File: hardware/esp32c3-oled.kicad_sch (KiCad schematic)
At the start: 2 parts, among them U1 ESP32-C3-WROOM-02

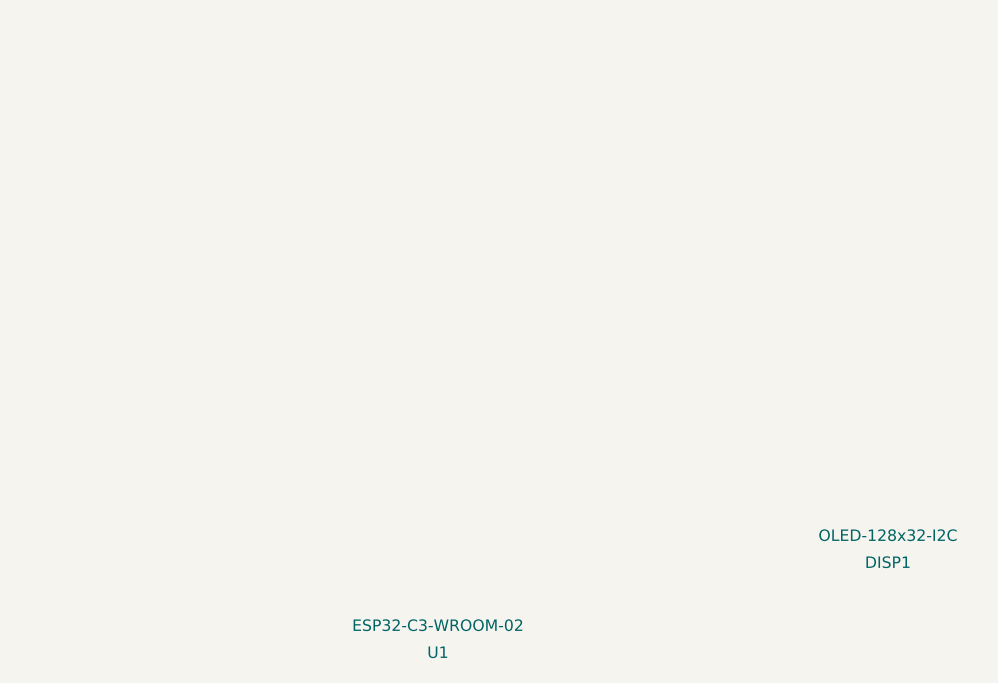
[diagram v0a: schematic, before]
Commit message: Update KiCad files
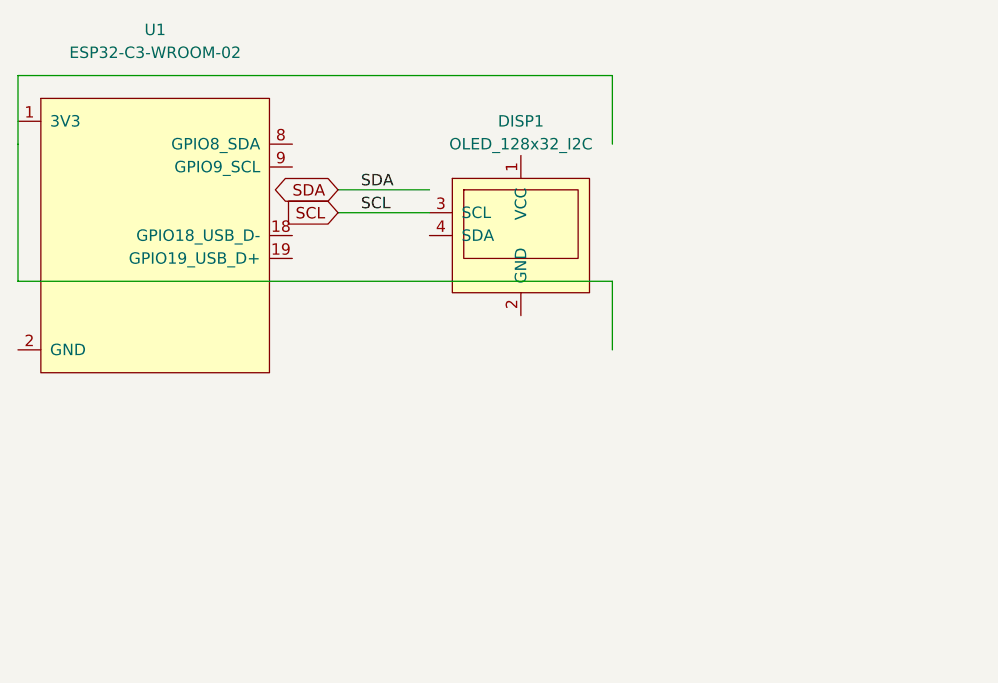
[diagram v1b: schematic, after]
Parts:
- DISP1: value OLED-128x32-I2C -> OLED_128x32_I2C; symbol Display_Character:OLED-128x32-I2C -> Display:OLED_128x32_I2C
- U1: symbol MCU_Module:ESP32-C3-WROOM-02 -> ESP32-C3:ESP32-C3-WROOM-02
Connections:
- new net SCL: DISP1.3 (SCL)
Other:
- title: (none) -> ESP32-C3 OLED Display - LCD4Linux
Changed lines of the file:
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@@
-(kicad_sch (version 20211123) (generator eeschema)
+(kicad_sch (version 20230121) (generator eeschema)
   (paper "A4")
-  (title "ESP32-C3 OLED Display - LCD4Linux")
-  (date "2026-03-09")
-  (rev "1.0")
-  (company "")
-  (comment 1 "128x32 I2C OLED with ESP32-C3")
-  (comment 2 "USB Serial communication for LCD4Linux")
-  (comment 3 "")
-  (comment 4 "")
-  (symbol (lib_id "MCU_Module:ESP32-C3-WROOM-02") (at 100 100 0) (unit 1)
-    (in_bom yes) (on_board yes)
-    (property "Reference" "U1" (id 0) (at 100 120 0))
-    (property "Value" "ESP32-C3-WROOM-02" (id 1) (at 100 117 0))
+  (title_block
+    (title "ESP32-C3 OLED Display - LCD4Linux")
+    (date "2026-03-12")
+    (rev "1.0")
+    (company "")
+    (comment 1 "128x32 I2C OLED with ESP32-C3")
+    (comment 2 "USB Serial communication for LCD4Linux")
+    (comment 3 "")
+    (comment 4 "")
   )
-  (symbol (lib_id "Display_Character:OLED-128x32-I2C") (at 150 100 0) (unit 1)
-    (in_bom yes) (on_board yes)
-    (property "Reference" "DISP1" (id 0) (at 150 110 0))
-    (property "Value" "OLED-128x32-I2C" (id 1) (at 150 107 0))
+  (wire (pts (xy 88.9 68.58) (xy 99.06 68.58))
+    (stroke (width 0) (type default))
+  )
+  (wire (pts (xy 88.9 71.12) (xy 99.06 71.12))
+    (stroke (width 0) (type default))
+  )
+  (wire (pts (xy 53.34 63.5) (xy 53.34 78.74))
+    (stroke (width 0) (type default))
+  )
+  (wire (pts (xy 119.38 78.74) (xy 119.38 86.36))
+    (stroke (width 0) (type default))
+  )
+  (wire (pts (xy 53.34 78.74) (xy 119.38 78.74))
+    (stroke (width 0) (type default))
+  )
+  (wire (pts (xy 53.34 55.88) (xy 53.34 63.5))
+    (stroke (width 0) (type default))
+  )
+  (wire (pts (xy 119.38 55.88) (xy 119.38 63.5))
+    (stroke (width 0) (type default))
+  )
+  (wire (pts (xy 53.34 55.88) (xy 119.38 55.88))
+    (stroke (width 0) (type default))
+  )
+  (label "SDA" (at 91.44 68.58 0) (fields_autoplaced)
+    (effects (font (size 1.27 1.27)) (justify left bottom))
+  )
+  (label "SCL" (at 91.44 71.12 0) (fields_autoplaced)
+    (effects (font (size 1.27 1.27)) (justify left bottom))
+  )
+  (global_label "SDA" (shape bidirectional) (at 88.9 68.58 180) (fields_autoplaced)
+    (effects (font (size 1.27 1.27)) (justify right))
+    (property "Intersheetrefs" "${INTERSHEET_REFS}" (at 82.6179 68.58 0)
+      (effects (font (size 1.27 1.27)) (justify right) hide)
+    )
+  )
+  (global_label "SCL" (shape input) (at 88.9 71.12 180) (fields_autoplaced)
+    (effects (font (size 1.27 1.27)) (justify right))
+    (property "Intersheetrefs" "${INTERSHEET_REFS}" (at 82.7993 71.12 0)
+      (effects (font (size 1.27 1.27)) (justify right) hide)
+    )
+  )
+  (symbol (lib_id "ESP32-C3:ESP32-C3-WROOM-02") (at 68.58 68.58 0) (unit 1)
+    (in_bom yes) (on_board yes) (dnp no)
+    (property "Reference" "U1" (at 68.58 50.8 0)
+      (effects (font (size 1.27 1.27)))
+    )
+    (property "Value" "ESP32-C3-WROOM-02" (at 68.58 53.34 0)
+      (effects (font (size 1.27 1.27)))
+    )
+    (property "Footprint" "" (at 68.58 68.58 0)
+      (effects (font (size 1.27 1.27)) hide)
+    )
+    (property "Datasheet" "" (at 68.58 68.58 0)
+      (effects (font (size 1.27 1.27)) hide)
+    )
+    (pin "1")
+    (pin "2")
+    (pin "8")
+    (pin "9")
+    (pin "18")
+    (pin "19")
+    (instances
+      (project "esp32c3-oled"
+        (path "/" (reference "U1") (unit 1))
+      )
+    )
+  )
+  (symbol (lib_id "Display:OLED_128x32_I2C") (at 109.22 71.12 0) (unit 1)
+    (in_bom yes) (on_board yes) (dnp no)
+    (property "Reference" "DISP1" (at 109.22 60.96 0)
+      (effects (font (size 1.27 1.27)))
+    )
+    (property "Value" "OLED_128x32_I2C" (at 109.22 63.5 0)
+      (effects (font (size 1.27 1.27)))
+    )
+    (property "Footprint" "" (at 109.22 71.12 0)
+      (effects (font (size 1.27 1.27)) hide)
+    )
+    (property "Datasheet" "" (at 109.22 71.12 0)
+      (effects (font (size 1.27 1.27)) hide)
+    )
+    (pin "1")
+    (pin "2")
+    (pin "3")
+    (pin "4")
+    (instances
+      (project "esp32c3-oled"
+        (path "/" (reference "DISP1") (unit 1))
+      )
+    )
   )
   (sheet_instances
     (path "/" (page "1"))
   )
-  (symbol_instances
-    (path "/11111111-2222-3333-4444-555555555555"
-      (reference "U1") (unit 1) (value "ESP32-C3-WROOM-02") (footprint "RF_Module:ESP32-C3-WROOM-02")
-    )
-    (path "/22222222-3333-4444-5555-666666666666"
-      (reference "DISP1") (unit 1) (value "OLED-128x32-I2C") (footprint "Display:OLED-128x32-I2C")
-    )
-  )
 )
